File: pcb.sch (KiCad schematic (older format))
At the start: 40 parts, among them J1 USB_B_Micro, J2 BAT, J3 Conn_01x07, J4 PROG, SW1 MultiDirectionSwitch_5way, SW2 M1, SW3 M2, SW4 SW_Push_SPDT, SW5 M3, SW6 RST, SW7 PGM, U1 MIC5219-3.3YMM, U2 ESP-12F, U3 PCF8574, U4 LTC4054

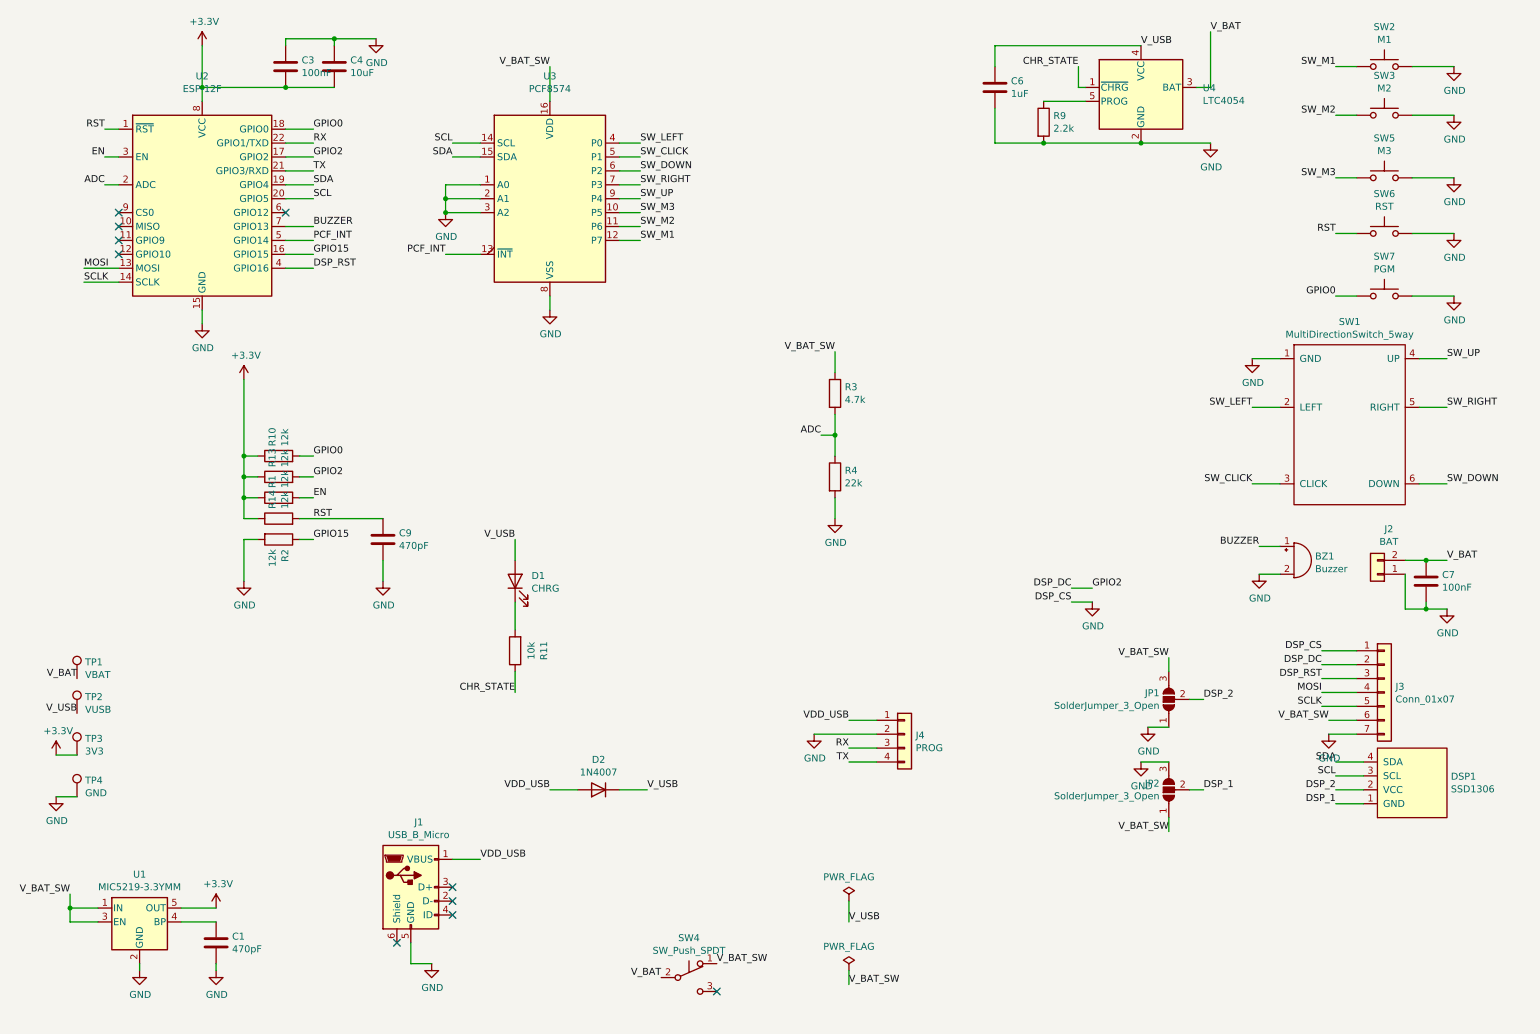
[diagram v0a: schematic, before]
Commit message: cleanup schematic
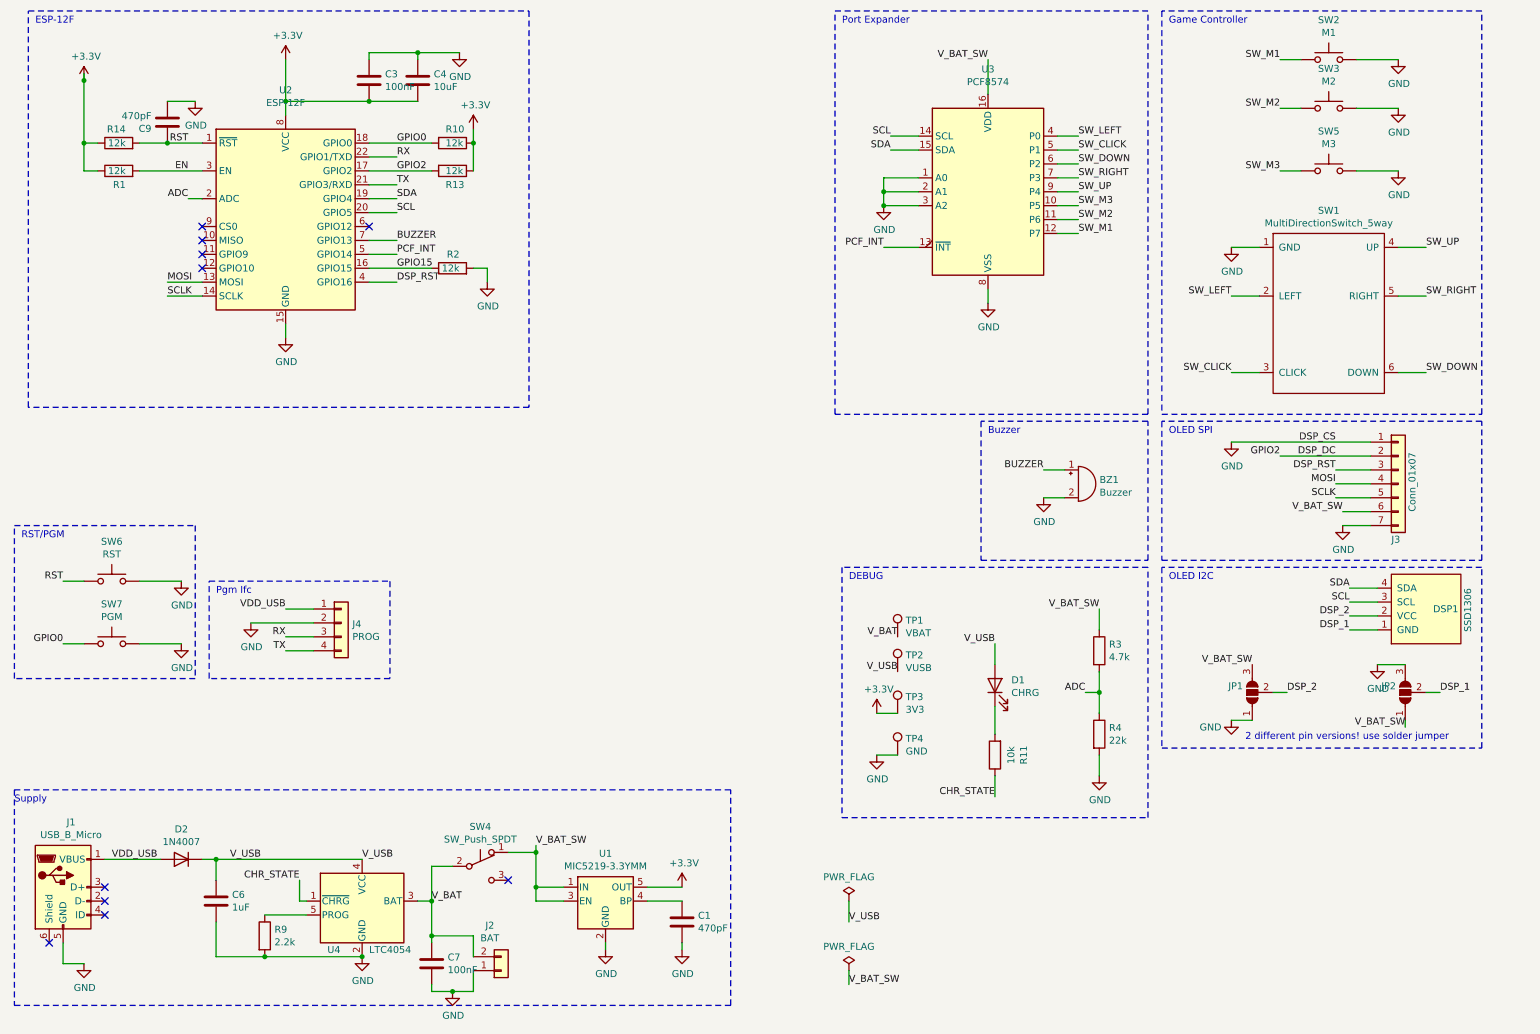
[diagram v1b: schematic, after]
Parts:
- JP1, JP2: value SolderJumper_3_Open -> (none)
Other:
- note added: "2 different pin versions! use solder jumper"
- note added: "Buzzer"
- note added: "DEBUG"
- note added: "ESP-12F"
- note added: "Game Controller"
- note added: "OLED I2C"
- note added: "OLED SPI"
- note added: "Pgm Ifc"
- note added: "Port Expander"
- note added: "RST/PGM"
- note added: "Supply"
- moved on the sheet: BZ1, C1, C3, C4, C6, C7, C9, D1, D2, DSP1, J1, J2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
